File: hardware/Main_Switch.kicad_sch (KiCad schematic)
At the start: 6 parts

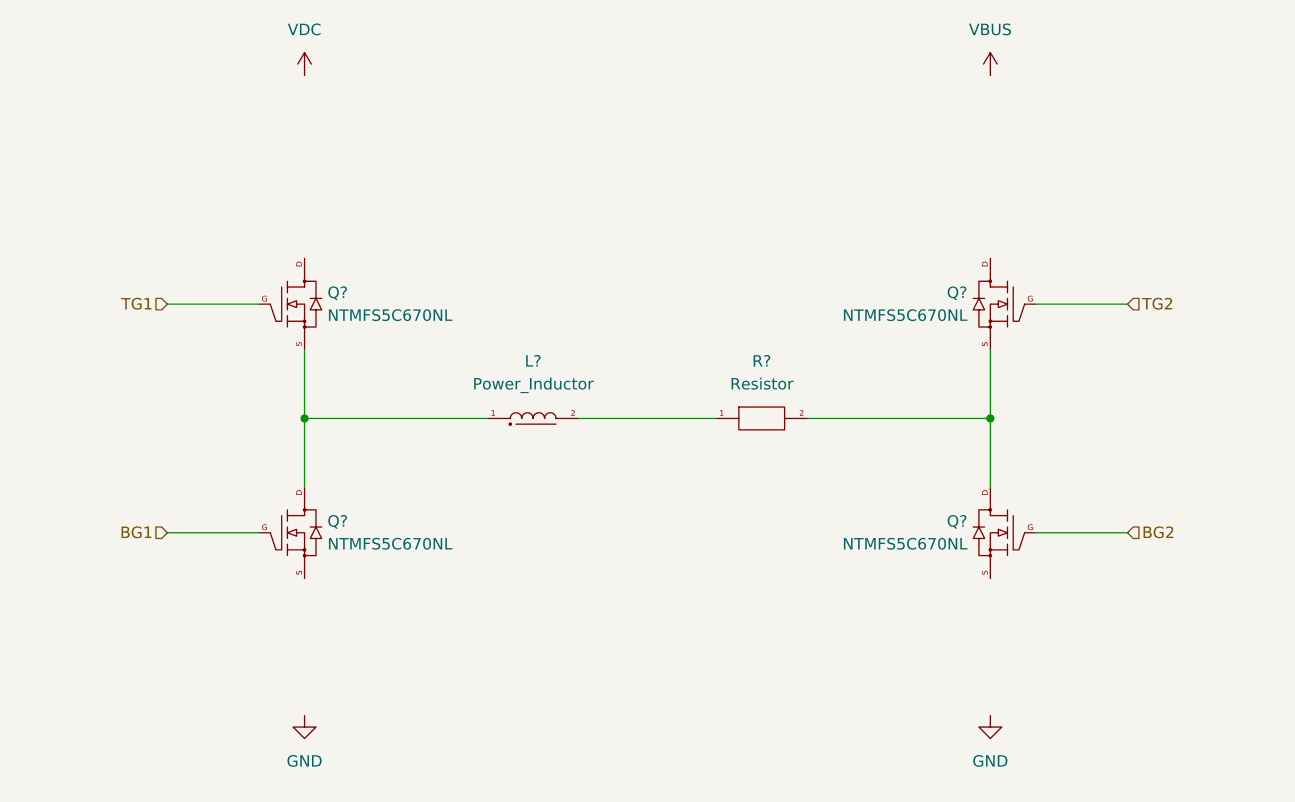
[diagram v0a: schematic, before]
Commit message: Nightly update
Update Driver and Main_Switch.
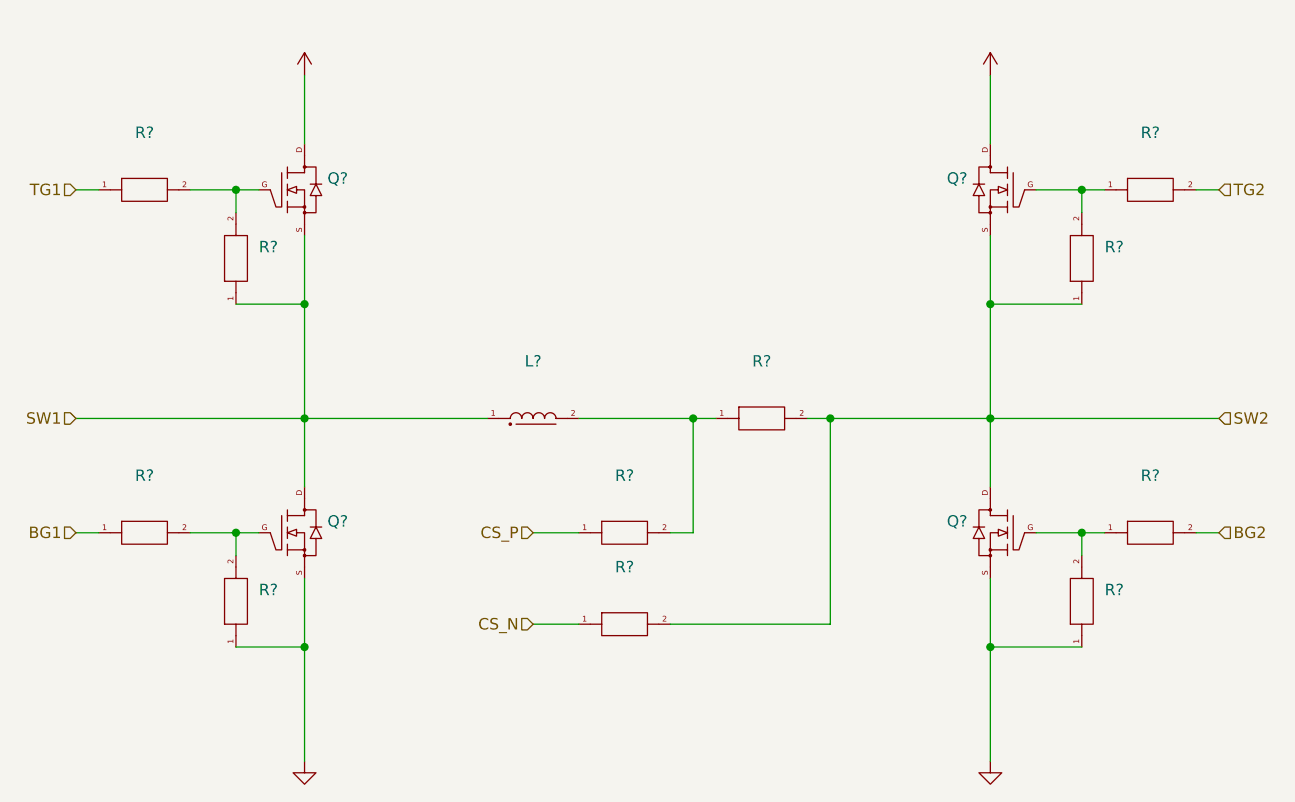
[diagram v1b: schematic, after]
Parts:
- added R? (x10): (no value), symbol Basic_passive_components:Resistor
- L?: value Power_Inductor -> (none)
- Q? (x4): value NTMFS5C670NL -> (none); footprint POWER_TRANSISTOR_SMD:SON-8_5x6_M -> (none)
- R?: value Resistor -> (none)
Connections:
- net BG1: now also R?.1; no longer Q?.G (Gate)
- net BG2: now also R?.2; no longer Q?.G (Gate)
- net GND: now also Q?.S (Source), Q?.S (Source), R?.1, R?.1
- net TG1: now also R?.1; no longer Q?.G (Gate)
- net TG2: now also R?.2; no longer Q?.G (Gate)
- net VBUS: now also Q?.D (Drain)
- net VDC: now also Q?.D (Drain)
- net SW2: now reaches Q?.D (Drain), Q?.S (Source), R?.2
- net SW2: now also R?.1, R?.2
- net SW1: now reaches L?.1, Q?.D (Drain), Q?.S (Source)
- net SW1: now also R?.1
- net at L?.2, R?.1: now also R?.2
- new net: Q?.G (Gate), R?.1, R?.2 (x2)
- new net: Q?.G (Gate), R?.2, R?.2 (x2)
- new net CS_N: R?.1
- new net CS_P: R?.1
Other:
- moved on the sheet: Q?
